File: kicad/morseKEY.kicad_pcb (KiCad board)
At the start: 2 copper layers, 50.8 x 17.8 mm, 16 parts, among them P1 USB_A, P2 KEY, P3 ISP, U1 ATTINY85-P

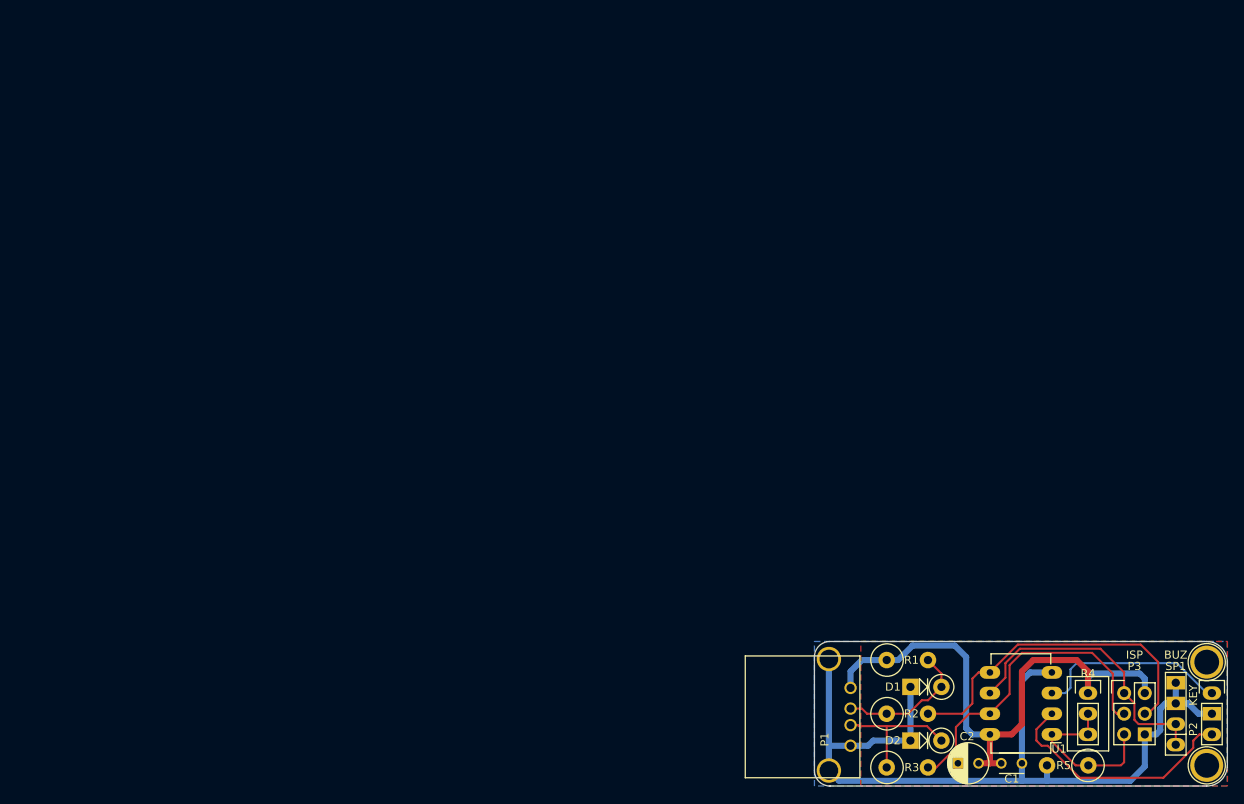
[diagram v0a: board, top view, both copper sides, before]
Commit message: board layout
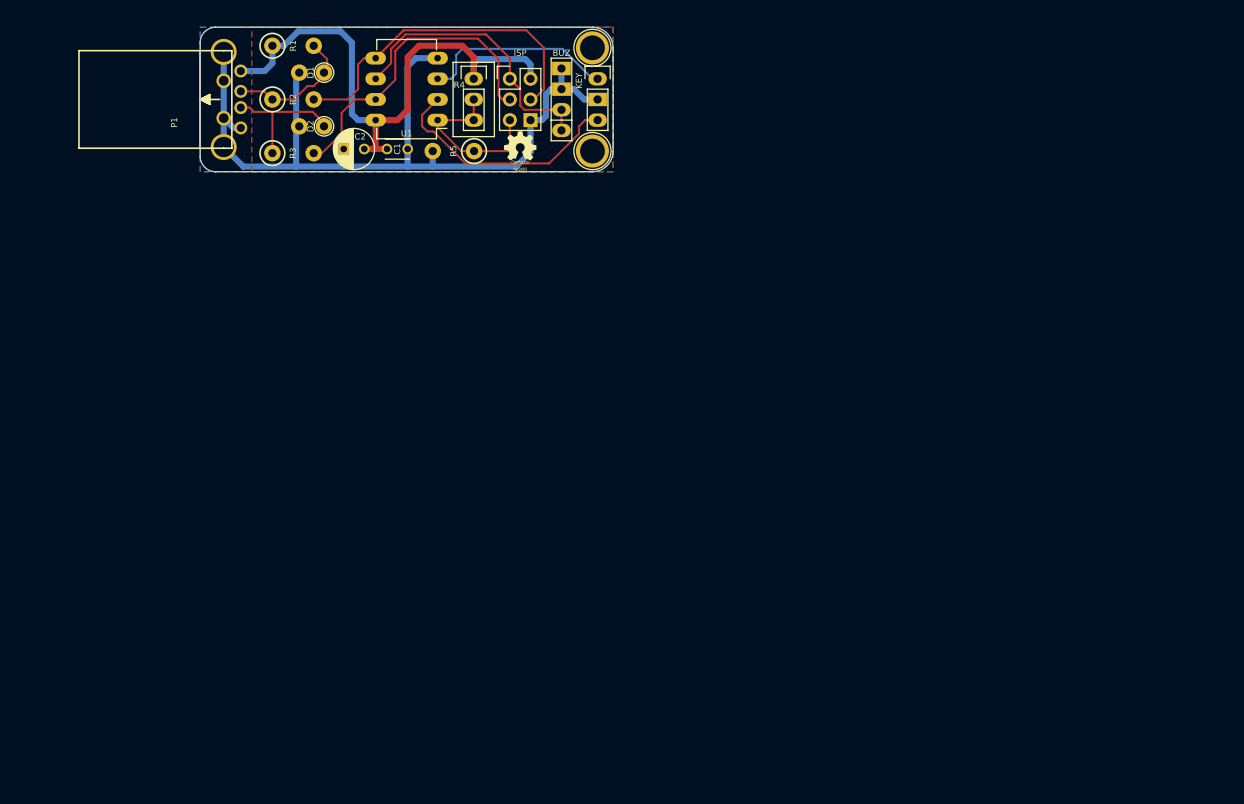
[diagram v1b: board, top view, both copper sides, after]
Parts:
- added G***: LOGO, morseKEY:morseKEY, B.Cu at (56.1, 34.8)
- added G***: LOGO, morseKEY:OSHW_logo_notext, F.Cu at (72.4, 41.3)
- D1, D2: footprint morseKEY:Diode_DO-41_SOD81_Vertical_KathodeUp -> morseKEY:Diode_DO-41_SOD81_Vertical_KathodeUp_2
- P1: footprint morseKEY:USB_A -> morseKEY:USB_A_up2-ah-th
- moved P1 107.9 mm to (33.0, 35.6)
- moved C1 106.9 mm to (57.3, 41.7)
- moved C2 106.9 mm to (51.9, 41.7)
- moved D1 106.9 mm to (46.7, 32.3)
- moved D2 106.9 mm to (46.7, 38.9)
- moved P3 106.9 mm to (72.4, 35.6)
- moved R1 106.9 mm to (44.5, 29.0)
- moved R2 106.9 mm to (44.5, 35.6)
- moved R3 106.9 mm to (44.5, 42.2)
- moved R4 106.9 mm to (66.7, 35.6)
- moved R5 106.9 mm to (64.2, 41.9)
- moved REF** 106.9 mm to (81.3, 41.9)
- moved REF** 106.9 mm to (81.3, 29.2)
- moved SP1 106.9 mm to (77.5, 35.6)
- moved U1 106.9 mm to (58.4, 34.3)
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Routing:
- net /GND: track 109.6 -> 104.2 mm
- net /5V: track 70.5 -> 69.9 mm
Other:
- board text added: "OpenSource Hardware"

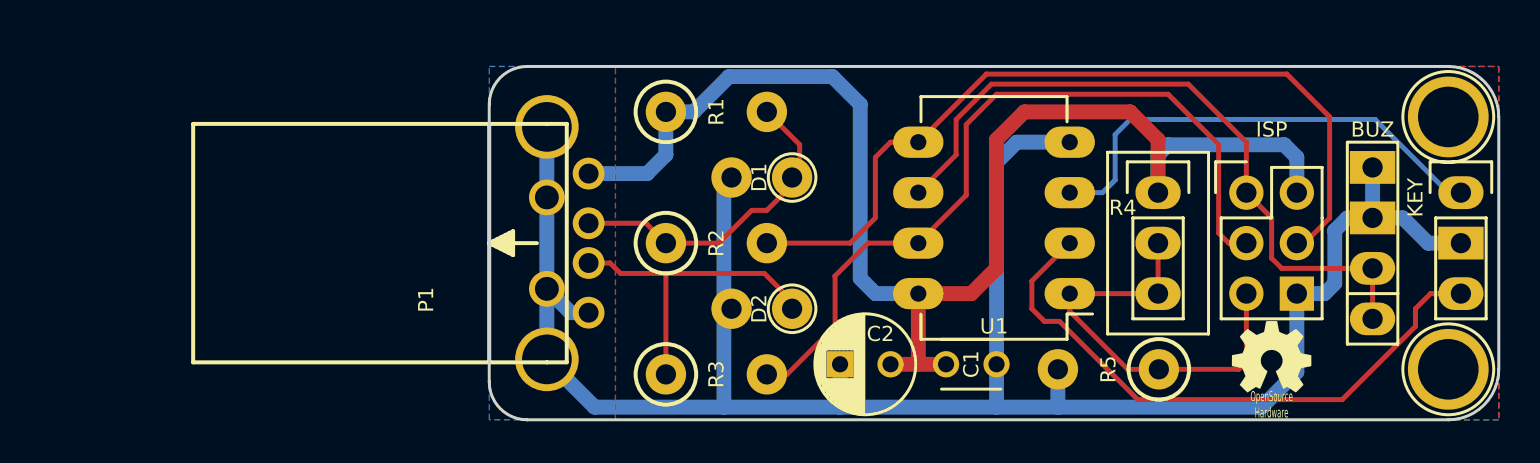
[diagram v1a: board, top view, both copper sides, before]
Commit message: gerbers
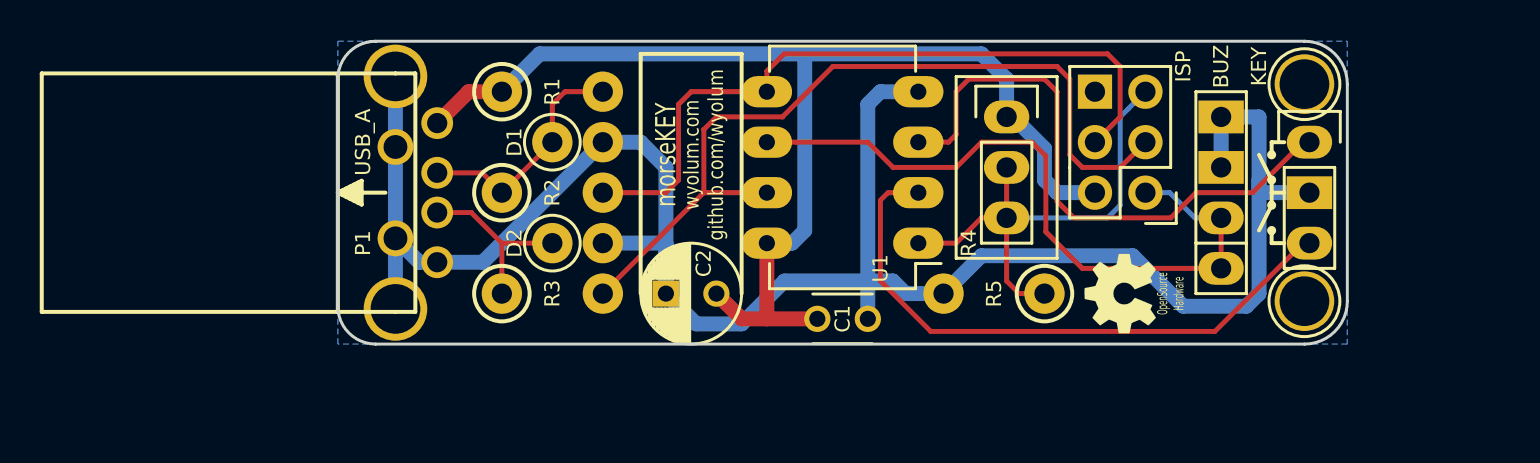
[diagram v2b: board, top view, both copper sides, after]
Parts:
- removed G***: LOGO, morseKEY:morseKEY
- removed REF** (x2): 1pin, Connect:1pin
- added G2: CKT, morseKEY:morseKEY, B.Cu at (49.5, 32.4)
- added P4: MTG, morseKEY:1pin, F.Cu at (74.0, 27.6)
- added P5: MTG, morseKEY:1pin, F.Cu at (74.0, 38.5)
- G1: renamed from G***; value LOGO -> OSHW-LOGO
- moved D2 9.84 mm to (37.5, 35.6), turned to 0 degrees
- moved C2 9.46 mm to (43.2, 38.1)
- moved D1 9.44 mm to (37.5, 30.5), turned to 0 degrees
- moved R3 9.20 mm to (36.2, 38.1)
- moved P3 9.16 mm to (64.8, 30.5), turned to 180 degrees
- moved R2 8.64 mm to (36.2, 33.0)
- moved R4 8.52 mm to (59.1, 31.8)
- moved R1 8.32 mm to (36.2, 27.9)
- moved G1 8.26 mm to (64.8, 38.1), turned to 90 degrees
- moved P1 8.03 mm to (25.4, 33.0)
- moved P2 8.03 mm to (74.3, 33.0)
- moved SP1 8.03 mm to (69.8, 33.0)
- moved U1 8.03 mm to (50.8, 31.8)
- moved R5 6.90 mm to (58.4, 38.1)
- moved C1 6.87 mm to (50.8, 39.4)
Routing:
- net /5V: track 69.9 -> 60.0 mm
- net /D+: track 16.7 -> 8.97 mm
- net /K1: track 24.1 -> 30.0 mm
- net /MOSI: track 41.8 -> 36.4 mm
- net /D-: track 16.4 -> 12.0 mm
- net /RST: track 21.7 -> 25.1 mm
- net /SCK: track 39.2 -> 41.9 mm
- net /GND: track 104.2 -> 104.8 mm
- removed copper zone on F.Cu, net /5V
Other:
- board size 50.8 x 17.8 mm -> 50.8 x 15.2 mm
- board text added: "forked from : mitxela.com/projects/morse_code_usb_keyboard_mk_ii"
- board text added: "morseKEY"
- board text added: "wyolum.com github.com/wyolum"

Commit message: BoM
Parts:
- R4: value 2k5 -> 1k5
- R5: value 2k5 -> 3k3
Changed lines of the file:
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@@
     (links 38)
     (no_connects 0)
-    (area 10.199999 23.536 88.007144 47.15)
+    (area 25.324999 25.324999 76.275001 40.715001)
     (thickness 1.6)
     (drawings 44)
@@
     (pad_to_mask_clearance 0.2)
     (aux_axis_origin 0 0)
-    (visible_elements FFFFEFFF)
+    (visible_elements FFFFFF7F)
     (pcbplotparams
       (layerselection 0x00030_00000000)
@@
     (pad 6 thru_hole rect (at 1.27 2.54 180) (size 1.7272 1.7272) (drill 1.016) (layers *.Cu *.Mask F.SilkS)
       (net 2 /GND))
-    (model header_2x3_TH_2_54mm.wrl
-      (at (xyz 0 0 0))
-      (scale (xyz 1 1 1))
-      (rotate (xyz 0 0 90))
-    )
   )
   (module morseKEY:C_Radial_D5_L6_P2.5 (layer F.Cu)
@@
     (pad 4 thru_hole rect (at 3.81 0 90) (size 1.651 2.286) (drill 1.016) (layers *.Cu *.Mask F.SilkS)
       (net 2 /GND))
-    (model header_1x4_TH_2_54mm.wrl
+    (model PS1240P02BT.wrl
       (at (xyz 0 0 0))
       (scale (xyz 1 1 1))
@@
     (pad 3 thru_hole oval (at 0 2.54) (size 2.286 1.651) (drill 1.016) (layers *.Cu *.Mask F.SilkS)
       (net 6 /K3))
-    (model header_1x3_TH_2_54mm.wrl
+    (model header_Male_RA_Low_3Pin.wrl
       (at (xyz 0 0 0))
       (scale (xyz 1 1 1))
@@
       (effects (font (size 0.762 0.762) (thickness 0.127)))
     )
-    (fp_text value 2k5 (at 0 -5.64) (layer F.Fab) hide
+    (fp_text value 1k5 (at 0 -5.64) (layer F.Fab) hide
       (effects (font (size 0.762 0.762) (thickness 0.127)))
     )
@@
       (effects (font (size 0.762 0.762) (thickness 0.127)))
     )
-    (fp_text value 2k5 (at -2.54 0.254 180) (layer F.SilkS) hide
-      (effects (font (size 0.762 0.762) (thickness 0.127)))
-    )
+    (fp_text value 3k3 (at -2.54 0.254 180) (layer F.SilkS) hide
+      (effects (font (size 0.762 0.762) (thickness 0.127)))
+    )
